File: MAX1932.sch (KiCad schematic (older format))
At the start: 23 parts, among them Q1 BSS123L, U5 MAX1932

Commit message: -5v supply, fpga routed
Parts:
- removed JP1, JP3: CAL, Jumper:SolderJumper-2_P1.3mm_Open_RoundedPad1.0x1.5mm, symbol Jumper:SolderJumper_2_Open
- removed R1: 100K, Resistor_SMD:R_0805_2012Metric, symbol Device:R_US
- removed R47: 10K, Resistor_SMD:R_0805_2012Metric, symbol Device:R_US
- removed TP2: DIV_A, TestPoint:TestPoint_THTPad_1.5x1.5mm_Drill0.7mm, symbol Connector:TestPoint
- removed TP3: DIV_B, TestPoint:TestPoint_THTPad_1.5x1.5mm_Drill0.7mm, symbol Connector:TestPoint
- removed TP4: DIV_C, TestPoint:TestPoint_THTPad_1.5x1.5mm_Drill0.7mm, symbol Connector:TestPoint
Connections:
- wire segments 59 -> 48
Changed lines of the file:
@@
 Wire Wire Line
 	4100 3300 4050 3300
-Text HLabel 8350 2350 2    50   Input ~ 0
+Text HLabel 7950 2350 2    50   Input ~ 0
 HV
 $Comp
@@
 	7450 2350 7550 2350
 $Comp
-L Jumper:SolderJumper_2_Open JP1
-U 1 1 5C3A13C0
-P 8000 2500
-F 0 "JP1" V 7954 2568 50  0000 L CNN
-F 1 "CAL" V 8045 2568 50  0000 L CNN
-F 2 "Jumper:SolderJumper-2_P1.3mm_Open_RoundedPad1.0x1.5mm" H 8000 2500 50  0001 C CNN
-F 3 "~" H 8000 2500 50  0001 C CNN
-	1    8000 2500
-	0    1    1    0
-$EndComp
-$Comp
-L Connector:TestPoint TP2
-U 1 1 5C3A15B3
-P 8350 2700
-F 0 "TP2" V 8545 2774 50  0000 C CNN
-F 1 "DIV_A" V 8454 2774 50  0000 C CNN
-F 2 "TestPoint:TestPoint_THTPad_1.5x1.5mm_Drill0.7mm" H 8550 2700 50  0001 C CNN
-F 3 "~" H 8550 2700 50  0001 C CNN
-	1    8350 2700
-	0    1    1    0
-$EndComp
-$Comp
-L Device:R_US R?
-U 1 1 5C3A1669
-P 8000 2900
-AR Path="/5C3A1669" Ref="R?"  Part="1"
-AR Path="/5C210B26/5C3A1669" Ref="R1"  Part="1"
-F 0 "R1" V 7795 2900 50  0000 C CNN
-F 1 "100K" V 7886 2900 50  0000 C CNN
-F 2 "Resistor_SMD:R_0805_2012Metric" V 8040 2890 50  0001 C CNN
-F 3 "~" H 8000 2900 50  0001 C CNN
-	1    8000 2900
-	-1   0    0    1
-$EndComp
-$Comp
-L Device:R_US R?
-U 1 1 5C3A16C7
-P 8000 3300
-AR Path="/5C3A16C7" Ref="R?"  Part="1"
-AR Path="/5C210B26/5C3A16C7" Ref="R47"  Part="1"
-F 0 "R47" V 7795 3300 50  0000 C CNN
-F 1 "10K" V 7886 3300 50  0000 C CNN
-F 2 "Resistor_SMD:R_0805_2012Metric" V 8040 3290 50  0001 C CNN
-F 3 "~" H 8000 3300 50  0001 C CNN
-	1    8000 3300
-	-1   0    0    1
-$EndComp
-$Comp
-L Jumper:SolderJumper_2_Open JP3
-U 1 1 5C3A3B39
-P 8000 3700
-F 0 "JP3" V 7954 3768 50  0000 L CNN
-F 1 "CAL" V 8045 3768 50  0000 L CNN
-F 2 "Jumper:SolderJumper-2_P1.3mm_Open_RoundedPad1.0x1.5mm" H 8000 3700 50  0001 C CNN
-F 3 "~" H 8000 3700 50  0001 C CNN
-	1    8000 3700
-	0    1    1    0
-$EndComp
-$Comp
-L Connector:TestPoint TP4
-U 1 1 5C3A14B5
-P 7900 3500
-F 0 "TP4" V 8100 3600 50  0000 C CNN
-F 1 "DIV_C" V 8000 3600 50  0000 C CNN
-F 2 "TestPoint:TestPoint_THTPad_1.5x1.5mm_Drill0.7mm" H 8100 3500 50  0001 C CNN
-F 3 "~" H 8100 3500 50  0001 C CNN
-	1    7900 3500
-	0    -1   -1   0
-$EndComp
-Wire Wire Line
-	8000 3550 8000 3500
-Wire Wire Line
-	7900 3500 8000 3500
-Connection ~ 8000 3500
-Wire Wire Line
-	8000 3500 8000 3450
-Wire Wire Line
-	8000 2650 8000 2700
-$Comp
 L Connector:TestPoint TP1
 U 1 1 5C3A155F
@@
 	1    0    0    -1
 $EndComp
-$Comp
-L power:GND #PWR?
-U 1 1 5C3B0B11
-P 8000 3900
-AR Path="/5C3B0B11" Ref="#PWR?"  Part="1"
-AR Path="/5C210B26/5C3B0B11" Ref="#PWR0105"  Part="1"
-F 0 "#PWR0105" H 8000 3650 50  0001 C CNN
-F 1 "GND" H 8005 3727 50  0000 C CNN
-F 2 "" H 8000 3900 50  0001 C CNN
-F 3 "" H 8000 3900 50  0001 C CNN
-	1    8000 3900
-	1    0    0    -1
-$EndComp
-Wire Wire Line
-	8000 3900 8000 3850
 Wire Wire Line
 	7550 2350 7750 2350
 Connection ~ 7550 2350
-Wire Wire Line
-	7750 2350 8000 2350
 Connection ~ 7750 2350
 Wire Wire Line
-	8000 2350 8350 2350
-Connection ~ 8000 2350
-$Comp
-L Connector:TestPoint TP3
-U 1 1 5C3A15F5
-P 7900 3100
-F 0 "TP3" V 8095 3174 50  0000 C CNN
-F 1 "DIV_B" V 8004 3174 50  0000 C CNN
-F 2 "TestPoint:TestPoint_THTPad_1.5x1.5mm_Drill0.7mm" H 8100 3100 50  0001 C CNN
-F 3 "~" H 8100 3100 50  0001 C CNN
-	1    7900 3100
-	0    -1   -1   0
-$EndComp
-Wire Wire Line
-	7900 3100 8000 3100
-Wire Wire Line
-	8000 3150 8000 3100
-Wire Wire Line
-	8350 2700 8000 2700
-Connection ~ 8000 2700
-Wire Wire Line
-	8000 2700 8000 2750
-Wire Wire Line
-	8000 3050 8000 3100
-Connection ~ 8000 3100
+	7750 2350 7950 2350
 $EndSCHEMATC

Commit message: routing only PI side left
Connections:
- net labels added: +5V
- net labels removed: VBUS
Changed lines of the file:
@@
 	5500 2350 5500 2400
-$Comp
-L power:VBUS #PWR?
-U 1 1 5C210D83
-P 5500 1850
-AR Path="/5C210D83" Ref="#PWR?"  Part="1"
-AR Path="/5C210B26/5C210D83" Ref="#PWR013"  Part="1"
-F 0 "#PWR013" H 5500 1700 50  0001 C CNN
-F 1 "VBUS" H 5515 2023 50  0000 C CNN
-F 2 "" H 5500 1850 50  0001 C CNN
-F 3 "" H 5500 1850 50  0001 C CNN
-	1    5500 1850
-	1    0    0    -1
-$EndComp
-Wire Wire Line
-	5500 1850 5500 1900
 $Comp
 L Device:C C?
@@
 Wire Wire Line
 	7750 2350 7950 2350
+$Comp
+L power:+5V #PWR?
+U 1 1 5C3A857A
+P 5500 1800
+F 0 "#PWR?" H 5500 1650 50  0001 C CNN
+F 1 "+5V" H 5515 1973 50  0000 C CNN
+F 2 "" H 5500 1800 50  0001 C CNN
+F 3 "" H 5500 1800 50  0001 C CNN
+	1    5500 1800
+	1    0    0    -1
+$EndComp
+Wire Wire Line
+	5500 1800 5500 1900
 $EndSCHEMATC

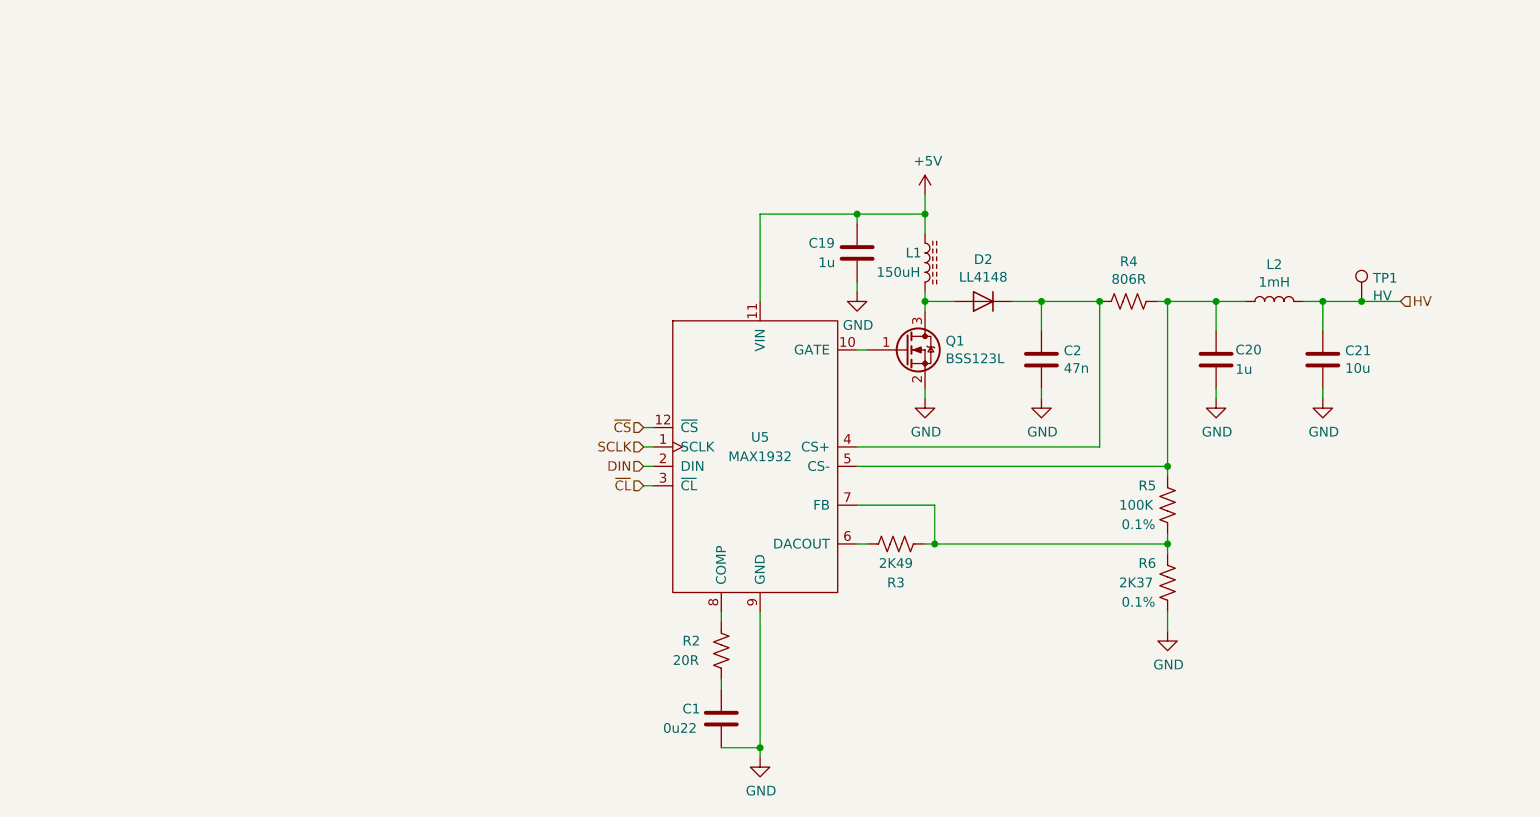
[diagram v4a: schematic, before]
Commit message: Finsihed layout for 1v2
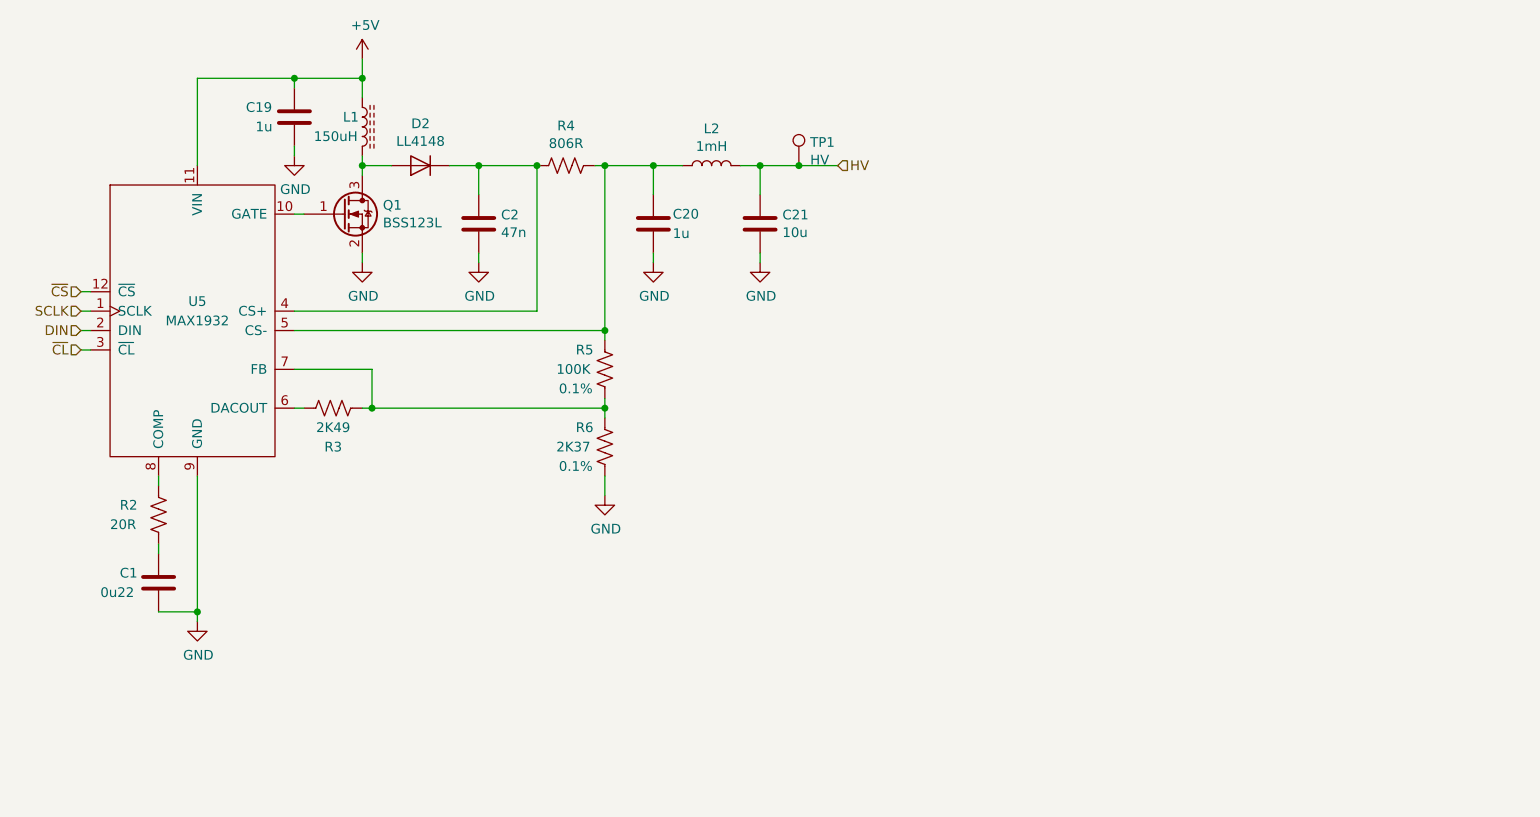
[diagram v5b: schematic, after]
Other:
- moved on the sheet: C1, C19, C2, C20, C21, D2, L1, L2, Q1, R2, R3, R4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
